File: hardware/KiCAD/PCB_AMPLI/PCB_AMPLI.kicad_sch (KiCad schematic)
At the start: 22 parts, among them J1 Conn_01x02, J2 Conn_01x02, J3 Conn_01x02, J4 Conn_01x02, J5 Conn_01x02, J6 Conn_01x02, J7 Conn_01x02, J8 Conn_01x02, SW1 SW_SPDT, SW2 SW_SPDT

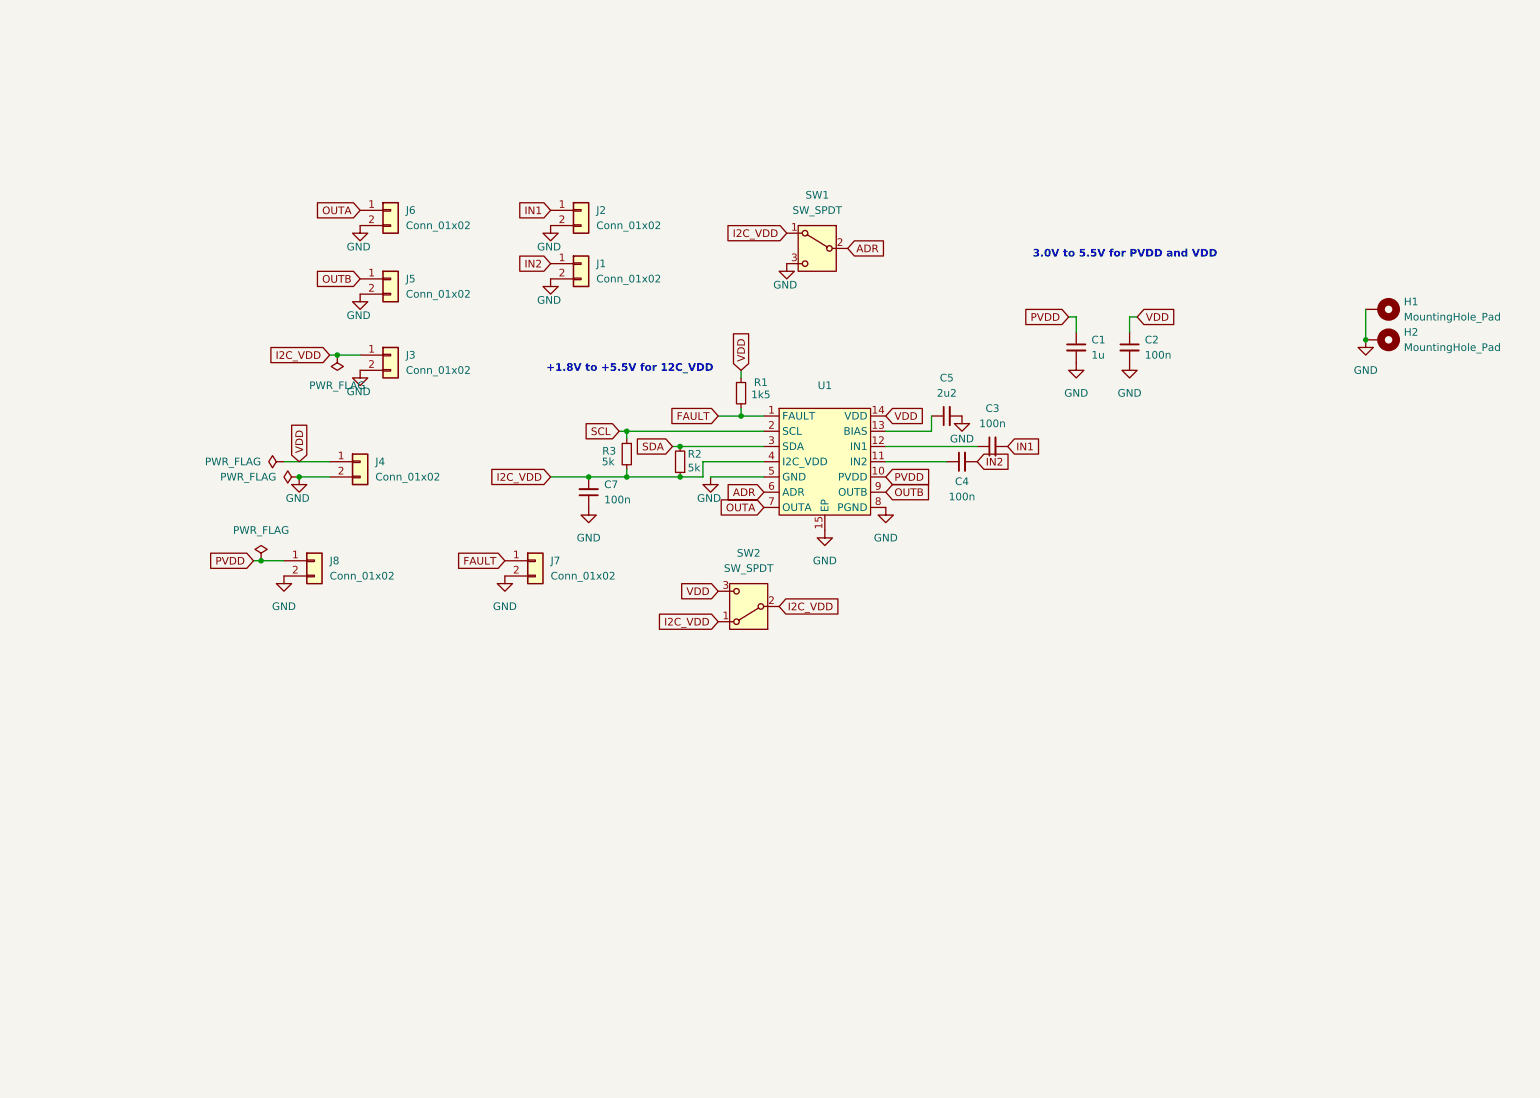
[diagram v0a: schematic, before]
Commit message: sch v2 ampli
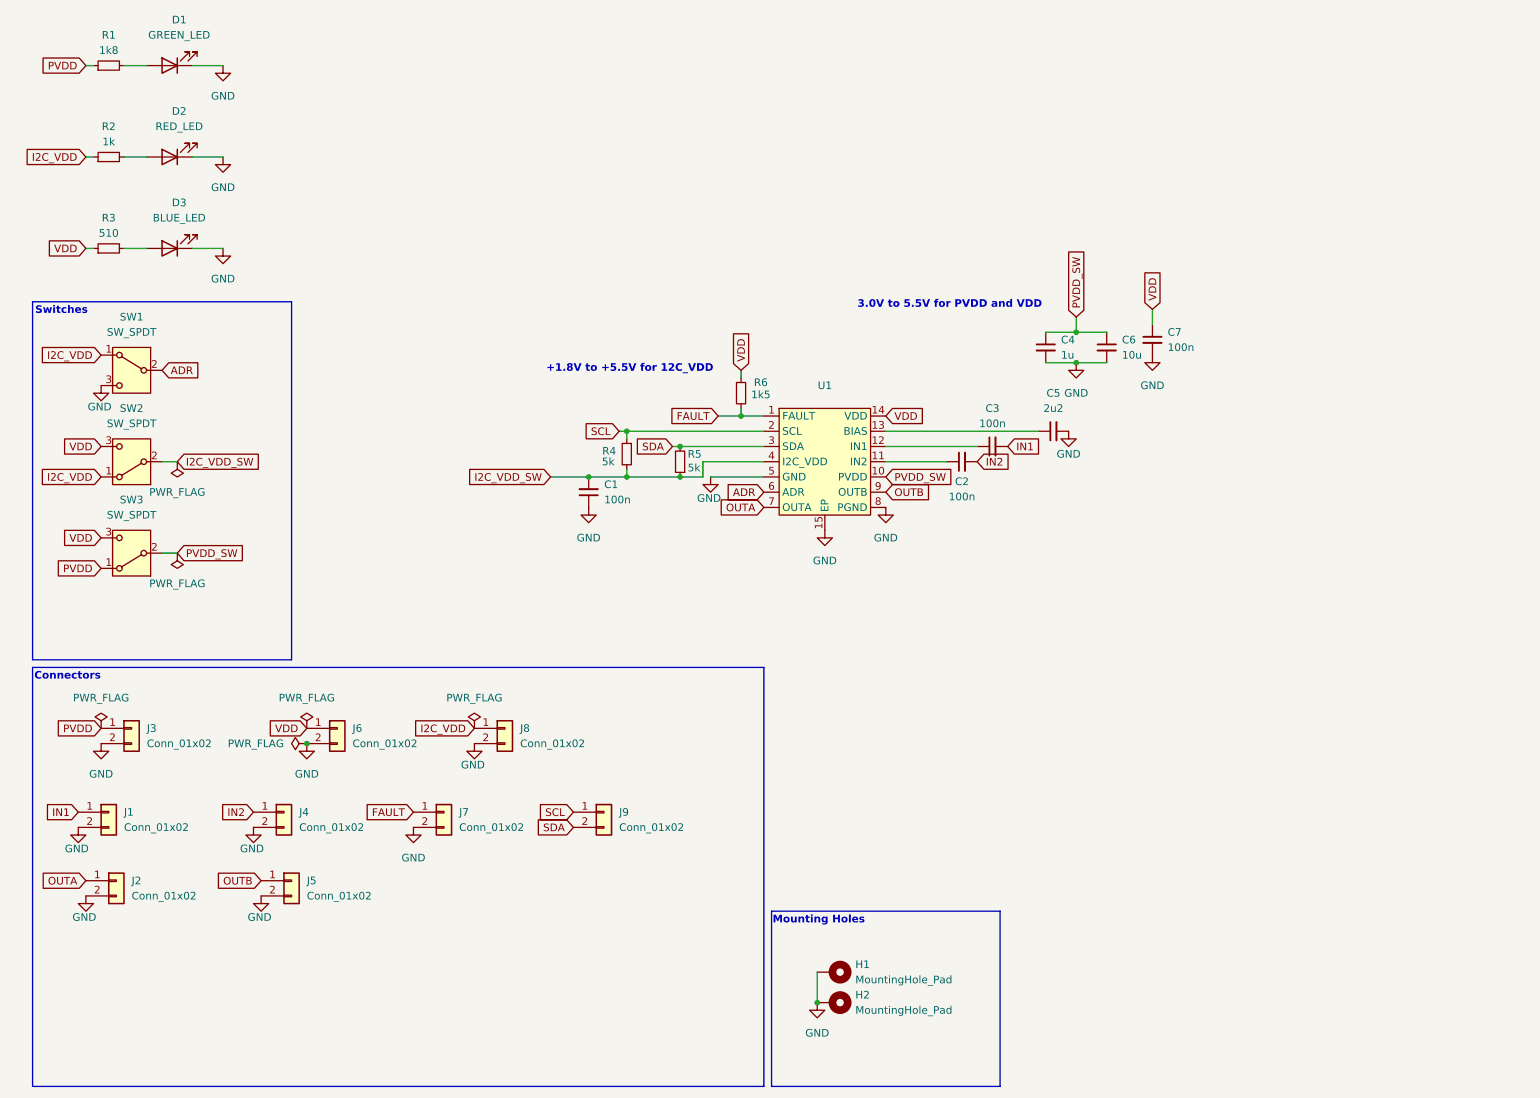
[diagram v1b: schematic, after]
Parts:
- added C6: 10u, Capacitor_SMD:C_0603_1608Metric, symbol Device:C_Small
- added D1: GREEN_LED, LED_SMD:LED_0603_1608Metric, symbol Device:LED
- added D2: RED_LED, LED_SMD:LED_0603_1608Metric, symbol Device:LED
- added D3: BLUE_LED, LED_SMD:LED_0603_1608Metric, symbol Device:LED
- added J9: Conn_01x02, Connector_PinHeader_2.54mm:PinHeader_1x02_P2.54mm_Vertical, symbol Connector_Generic:Conn_01x02
- added R1: 1k8, symbol Device:R_Small
- added R2: 1k, symbol Device:R_Small
- added R3: 510, symbol Device:R_Small
- added SW3: SW_SPDT, Personal:450406020024, symbol Switch:SW_SPDT
- U1: footprint Package_SO:HTSSOP-14-1EP_4.4x5mm_P0.65mm_EP3.4x5mm_Mask3x3.1mm -> (none); MPN LM48100QMHX/NOPB -> (none)
- renumbered C7 to C1, C4 to C2, C1 to C4, C2 to C7, J2 to J1, J6 to J2, J8 to J3, J1 to J4, J4 to J6, J3 to J8, R3 to R4, R2 to R5, R1 to R6
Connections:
- net GND: now also C6.2, D1.1 (K), D2.1 (K), D3.1 (K)
- net I2C_VDD: now also R2.1; no longer C1.2, R4.2, R5.1, SW2.2 (B), U1.4 (I2C_VDD)
- net PVDD: now also R1.1, SW3.1 (A); no longer C4.1, U1.10 (PVDD)
- net SCL: now also J9.1 (Pin_1)
- net SDA: now also J9.2 (Pin_2)
- net VDD: now also R3.1, SW3.3 (C)
- new net: D3.2 (A), R3.2
- new net: D1.2 (A), R1.2
- new net: D2.2 (A), R2.2
- new net I2C_VDD_SW: C1.2, R4.2, R5.1, SW2.2 (B), U1.4 (I2C_VDD)
- new net PVDD_SW: C4.1, C6.1, SW3.2 (B), U1.10 (PVDD)
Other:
- note added: "Connectors"
- note added: "Mounting Holes"
- note added: "Switches"
- moved on the sheet: C4, C5, C7, H1, H2, J1, J2, J3, J4, J5, J6, J7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
